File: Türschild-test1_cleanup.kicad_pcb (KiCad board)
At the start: 2 copper layers, 90.2 x 76.2 mm, 84 parts, among them J1 Conn_01x03_Male, J3 USB_B_Micro, J4 Conn_01x24_MountingPin, Q3 Si1442DH, U1 BQ25570, U2 BQ27441-G1, U3 ESP32-WROOM-32, U4 CP2102N-A01-GQFN28

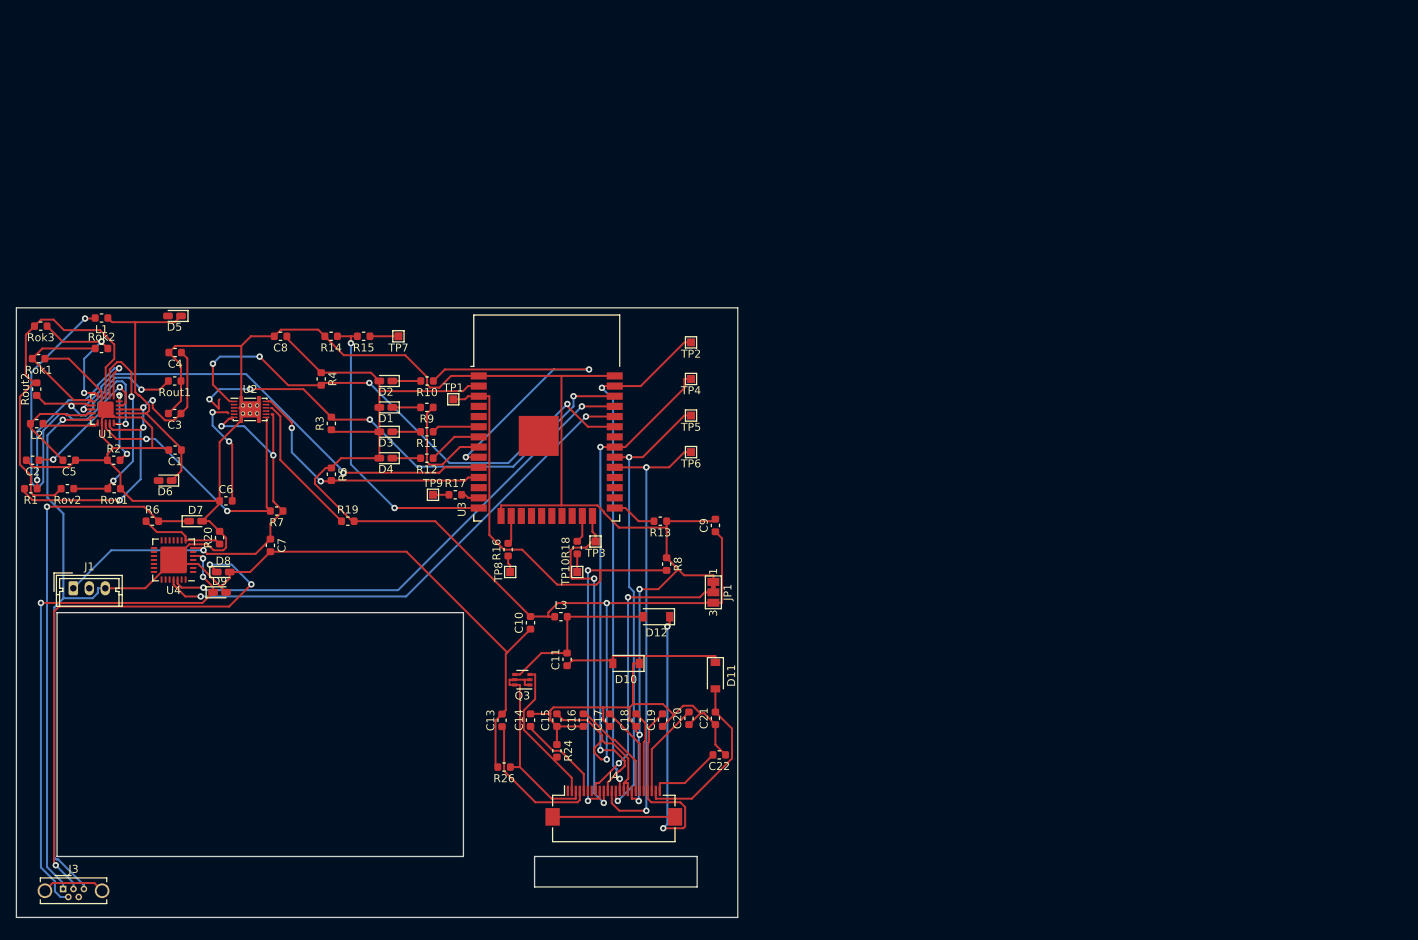
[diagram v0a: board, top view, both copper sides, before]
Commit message: HowTo Changes mit Daniel
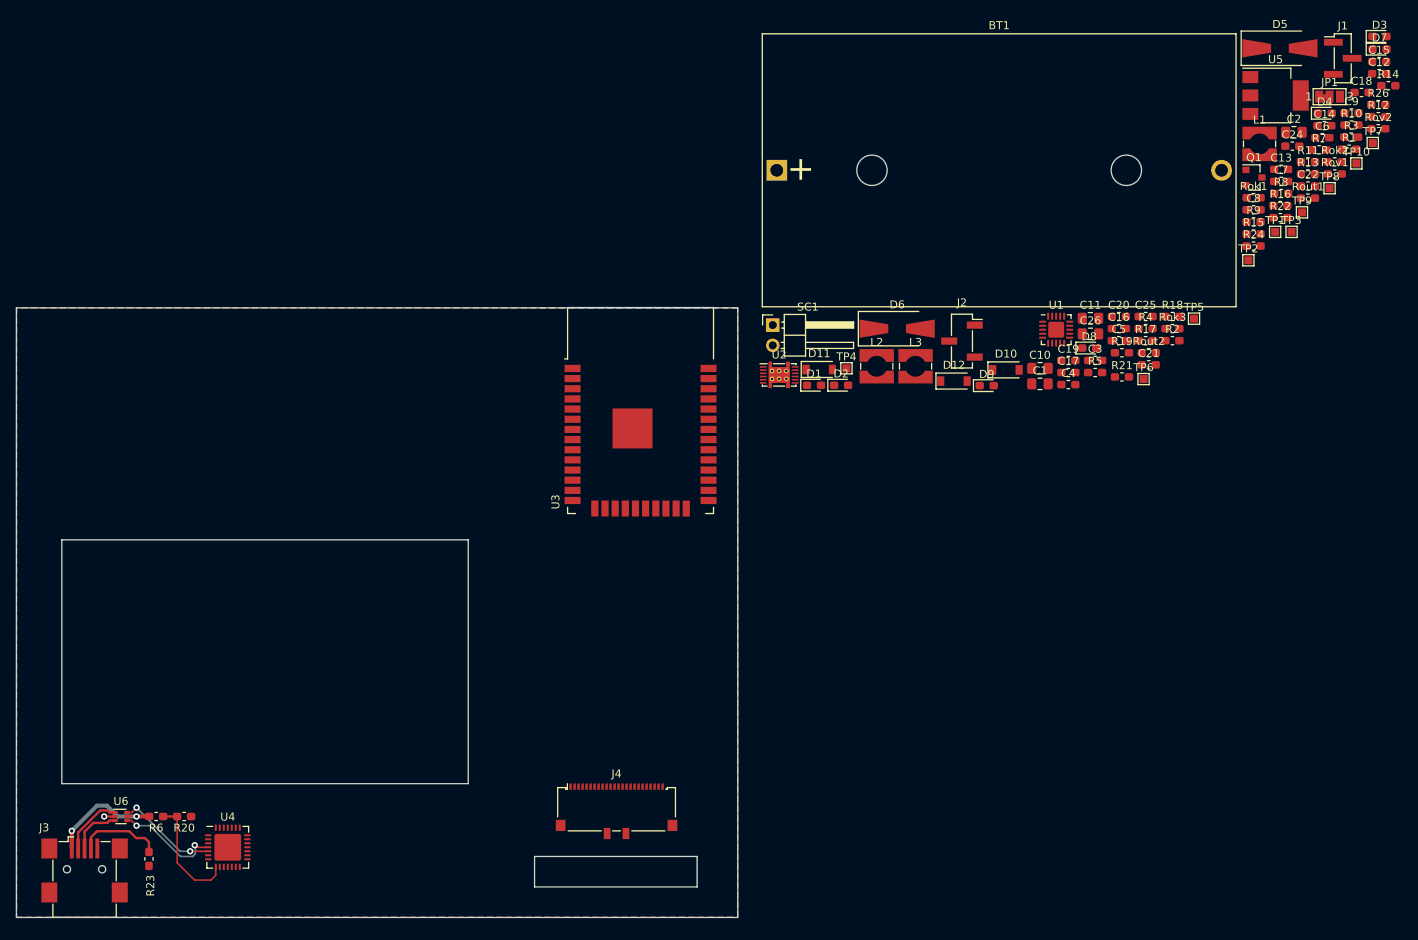
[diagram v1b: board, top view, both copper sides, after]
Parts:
- removed Q3: Si1442DH, Package_TO_SOT_SMD:SOT-363_SC-70-6
- added BT1: 3,7V, Battery:BatteryHolder_Bulgin_BX0036_1xC, F.Cu at (201.7, 34.9)
- added C12: 1µ, Capacitor_SMD:C_0603_1608Metric_Pad1.05x0.95mm_HandSolder, F.Cu at (277.0, 22.8)
- added C24: 100n, Capacitor_SMD:C_0603_1608Metric_Pad1.05x0.95mm_HandSolder, F.Cu at (266.2, 31.9)
- added C25: 100n, Capacitor_SMD:C_0603_1608Metric_Pad1.05x0.95mm_HandSolder, F.Cu at (247.8, 53.2)
- added C26: 4u7, Capacitor_SMD:C_0805_2012Metric_Pad1.15x1.40mm_HandSolder, F.Cu at (240.9, 55.3)
- added J2: Conn_01x03_Female, Connector_PinSocket_2.00mm:PinSocket_1x03_P2.00mm_Vertical_SMD_Pin1Right, F.Cu at (224.9, 56.2)
- added Q1: IRLML2502PbF, Package_TO_SOT_SMD:SOT-23, F.Cu at (261.4, 35.8)
- added R21: 0R, Resistor_SMD:R_0603_1608Metric_Pad1.05x0.95mm_HandSolder, F.Cu at (244.9, 60.7)
- added R22: 1K, Resistor_SMD:R_0603_1608Metric_Pad1.05x0.95mm_HandSolder, F.Cu at (264.7, 40.8)
- added R23: 4K7, Resistor_SMD:R_0603_1608Metric_Pad1.05x0.95mm_HandSolder, F.Cu at (123.2, 121.0)
- added SC1: Solar_Cells, Connector_PinHeader_2.54mm:PinHeader_1x02_P2.54mm_Horizontal, F.Cu at (201.2, 54.2)
- added U5: LM1117-3.3, Package_TO_SOT_SMD:SOT-223-3_TabPin2, F.Cu at (264.1, 25.5)
- added U6: WE-TVS-82400152, Package_TO_SOT_SMD:SOT-563, F.Cu at (119.8, 115.7)
- C1, C10, C11, C2: footprint Capacitor_SMD:C_0603_1608Metric -> Capacitor_SMD:C_0805_2012Metric_Pad1.15x1.40mm_HandSolder
- C13, C14, C15, C16, C17, C18, C19, C20, C21, C22, C5, C6, C7, C8, C9: footprint Capacitor_SMD:C_0603_1608Metric -> Capacitor_SMD:C_0603_1608Metric_Pad1.05x0.95mm_HandSolder
- C3, C4: value 0,1µF -> 100n; footprint Capacitor_SMD:C_0603_1608Metric -> Capacitor_SMD:C_0603_1608Metric_Pad1.05x0.95mm_HandSolder
- D1, D2, D3, D4: footprint LED_SMD:LED_0603_1608Metric_Castellated -> LED_SMD:LED_0603_1608Metric_Pad1.05x0.95mm_HandSolder
- D10, D11, D12: value MBR0530 -> MBR0530T1G
- D5, D6: value D_Schottky_Small -> SS16; footprint Diode_SMD:D_0603_1608Metric_Castellated -> Diode_SMD:D_SMA-SMB_Universal_Handsoldering
- D7, D8, D9: footprint Diode_SMD:D_0603_1608Metric_Castellated -> Diode_SMD:D_0603_1608Metric_Pad1.05x0.95mm_HandSolder
- J1: footprint Connector_Molex:Molex_Micro-Latch_53253-0370_1x03_P2.00mm_Vertical -> Connector_PinHeader_2.00mm:PinHeader_1x03_P2.00mm_Vertical_SMD_Pin1Left
- J3: footprint Connector_USB:USB_Micro-B_Wuerth_614105150721_Vertical_CircularHoles -> Connector_USB:USB_Mini-B_Wuerth_65100516121_Horizontal
- J4: footprint Connector_FFC-FPC:Hirose_FH12-24S-0.5SH_1x24-1MP_P0.50mm_Horizontal -> Connector_FFC-FPC:Molex_502244-2430_1x24-1MP_P0.5mm_Horizontal
- L1, L2, L3: footprint Inductor_SMD:L_0603_1608Metric -> Inductor_SMD:L_Wuerth_WE-TPC-3816
- R1, R10, R11, R12, R13, R14, R15, R16, R17, R18, R19, R2, R20, R24, R26, R3, R4, R5, R6, R7, R8, R9, Rok1, Rok2, Rok3, Rout1, Rout2, Rov1, Rov2: footprint Resistor_SMD:R_0603_1608Metric -> Resistor_SMD:R_0603_1608Metric_Pad1.05x0.95mm_HandSolder
- moved J1 172.0 mm to (272.5, 20.9)
- moved R1 170.2 mm to (273.3, 32.2), turned to 0 degrees
- moved Rov2 169.9 mm to (276.9, 29.7), turned to 0 degrees
- moved C2 162.9 mm to (266.4, 30.1), turned to 0 degrees
- moved D7 159.3 mm to (277.1, 19.7)
- moved Rov1 157.6 mm to (271.5, 35.3), turned to 0 degrees
- moved Rok2 155.9 mm to (271.5, 33.8)
- moved Rok1 153.2 mm to (261.3, 38.3), turned to 0 degrees
- moved L1 146.4 mm to (262.1, 31.6), turned to 0 degrees
- moved C6 144.4 mm to (269.9, 30.8)
- moved Rout1 143.5 mm to (268.1, 38.4), turned to 0 degrees
- moved D5 142.2 mm to (264.6, 19.6), turned to 0 degrees
- moved Rok3 141.5 mm to (251.2, 54.7), turned to 0 degrees
- moved Rout2 139.1 mm to (248.2, 57.7), turned to 0 degrees
- moved R7 137.9 mm to (269.5, 32.3), turned to 0 degrees
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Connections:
- D7 pad 1: Net-(D7-Pad1) -> VBUS
- J3 pad 1: Net-(D7-Pad1) -> VBUS
- J3 pad 2: Net-(D9-Pad1) -> Net-(J3-Pad2)
- J3 pad 3: Net-(D8-Pad1) -> Net-(J3-Pad3)
- J3 pad 6: Net-(J3-Pad6) -> GND
- R20 pad 1: Net-(R20-Pad1) -> GND
- R20 pad 2: GND -> Net-(R20-Pad2)
- R6 pad 1: Net-(R20-Pad1) -> Net-(R20-Pad2)
- R6 pad 2: Net-(D7-Pad1) -> VBUS
- U3 pad 27: Net-(U3-Pad27) -> USBID
- U3 pad 39: (no net) -> GND
- U4 pad 4: Net-(D8-Pad1) -> Net-(U4-Pad4)
- U4 pad 5: Net-(D9-Pad1) -> Net-(U4-Pad5)
- U4 pad 8: Net-(R20-Pad1) -> Net-(R20-Pad2)
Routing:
- net GND: track 476.0 -> 1.35 mm, vias 4 -> 1
- net +3V3: track 161.7 -> 0.00 mm, vias 2 -> 0
- net ESP_EN: track 81.2 -> 0.00 mm, vias 2 -> 0
- net Net-(D8-Pad1): track 69.2 -> 0.00 mm, vias 3 -> 0
- net Net-(D7-Pad1): track 67.1 -> 0.00 mm, vias 1 -> 0
- net Net-(D9-Pad1): track 66.9 -> 0.00 mm, vias 3 -> 0
- net SDA: track 66.5 -> 0.00 mm, vias 4 -> 0
- net ESP_CON_RX: track 65.7 -> 0.00 mm, vias 2 -> 0
- net ESP_CON_TX: track 65.0 -> 0.00 mm, vias 2 -> 0
- net ESP_MOSI: track 64.8 -> 0.00 mm, vias 2 -> 0
- net SCL: track 62.5 -> 0.00 mm, vias 4 -> 0
- net ESP_MISO: track 61.7 -> 0.00 mm, vias 2 -> 0
- net ESP_CS: track 59.5 -> 0.00 mm, vias 2 -> 0
- net VBAT_OK: track 58.2 -> 0.00 mm, vias 2 -> 0
- net ESP_SCK: track 57.1 -> 0.00 mm, vias 2 -> 0
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- added copper zone on B.Cu, net GND
- added copper zone on F.Cu, net GND
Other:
- outline, holes or cut-outs redrawn
- net class Default: clearance 0.2 -> 0.15; trace_width 0.25 -> 0.15
- rule trace_clearance: 0.2 -> 0.15
- rule trace_min: 0.2 -> 0.15

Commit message: Version 1
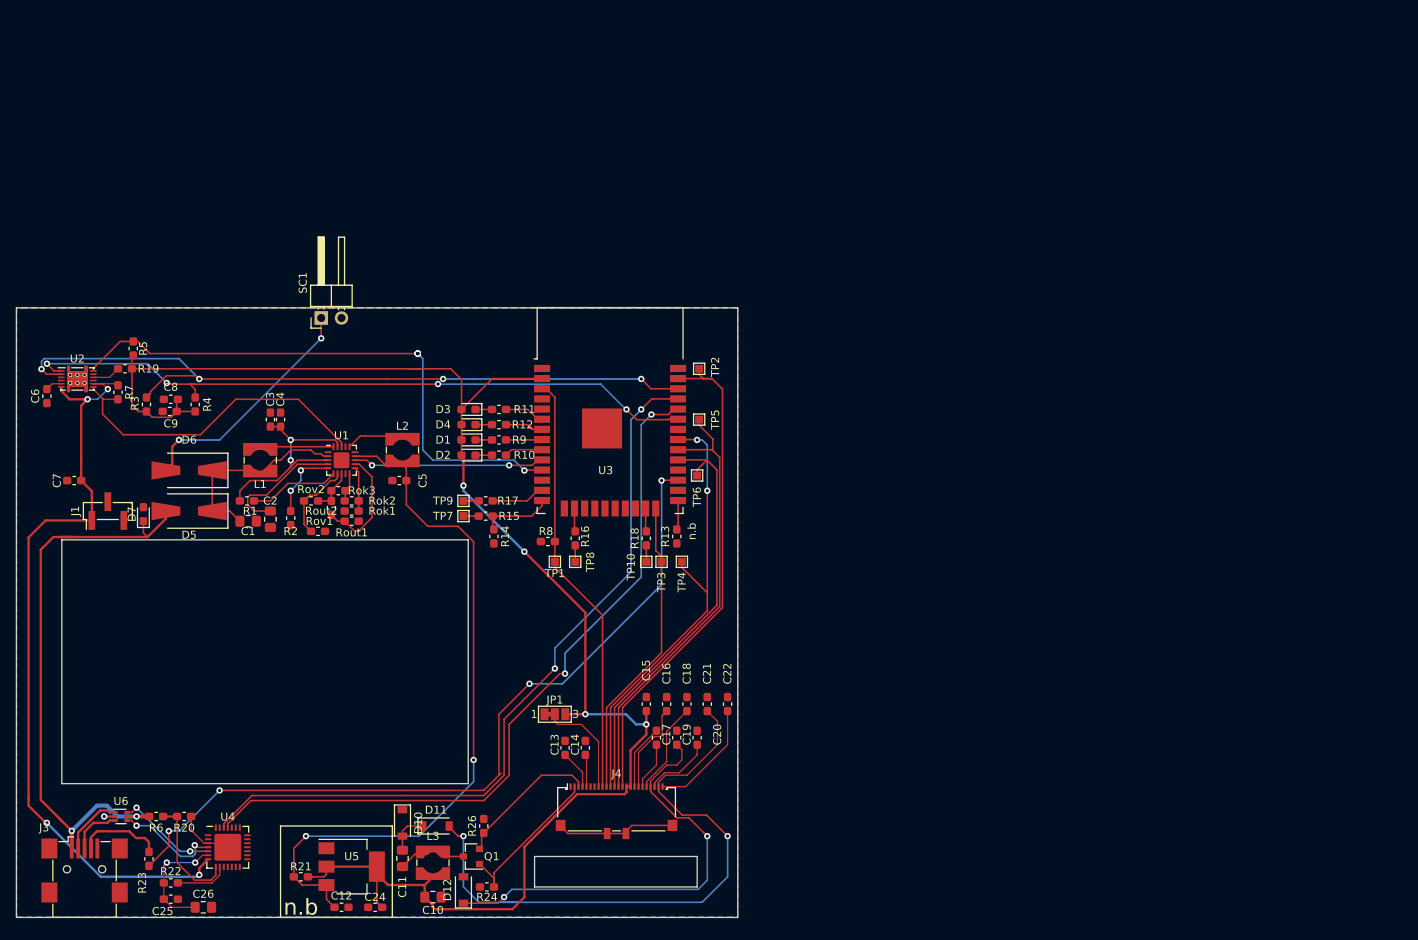
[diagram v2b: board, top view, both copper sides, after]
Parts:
- removed BT1: 3,7V, Battery:BatteryHolder_Bulgin_BX0036_1xC
- removed D8, D9: D_Schottky_Small, Diode_SMD:D_0603_1608Metric_Pad1.05x0.95mm_HandSolder
- removed J2: Conn_01x03_Female, Connector_PinSocket_2.00mm:PinSocket_1x03_P2.00mm_Vertical_SMD_Pin1Right
- moved C12 166.4 mm to (147.3, 127.0)
- moved D7 165.1 mm to (122.6, 77.9), turned to 90 degrees
- moved J1 164.4 mm to (118.1, 77.5), turned to 90 degrees
- moved C6 162.7 mm to (110.5, 63.1), turned to 90 degrees
- moved R22 161.7 mm to (126.0, 124.0)
- moved C7 155.4 mm to (113.9, 73.7), turned to 180 degrees
- moved R3 154.3 mm to (122.9, 64.1), turned to 90 degrees
- moved R7 153.2 mm to (119.4, 62.6), turned to 270 degrees
- moved C9 152.4 mm to (125.8, 65.0), turned to 180 degrees
- moved U5 150.4 mm to (148.6, 121.9)
- moved C24 149.0 mm to (151.5, 127.0), turned to 180 degrees
- moved D5 148.1 mm to (128.3, 77.5), turned to 180 degrees
- moved R1 144.6 mm to (135.5, 76.2), turned to 180 degrees
- moved R26 143.6 mm to (165.1, 116.8), turned to 90 degrees
- moved C25 142.0 mm to (126.0, 126.0)
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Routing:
- net +3V3: track 0.00 -> 203.9 mm, vias 0 -> 4
- net USBID: track 0.00 -> 99.7 mm, vias 0 -> 4
- net Net-(C7-Pad1): track 0.00 -> 98.2 mm, vias 0 -> 4
- net ESP_CON_TX: track 0.00 -> 96.0 mm, vias 0 -> 2
- net ESP_CON_RX: track 0.00 -> 94.6 mm, vias 0 -> 2
- net SCL: track 0.00 -> 93.0 mm, vias 0 -> 4
- net VCC: track 0.00 -> 89.1 mm, vias 0 -> 2
- net SDA: track 0.00 -> 86.9 mm, vias 0 -> 4
- net PREVGL: track 0.00 -> 77.3 mm, vias 0 -> 2
- net GPOUT: track 0.00 -> 71.2 mm, vias 0 -> 5
- net ESP_MOSI: track 0.00 -> 63.4 mm
- net VBUS: track 14.9 -> 74.2 mm
- net ESP_MISO: track 0.00 -> 56.8 mm, vias 0 -> 2
- net ESP_SCK: track 0.00 -> 56.6 mm
- net PREVGH: track 0.00 -> 55.0 mm, vias 0 -> 2
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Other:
- board text added: "n.b"
